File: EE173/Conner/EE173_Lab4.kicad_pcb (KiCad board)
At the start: 2 copper layers, 81.3 x 57.1 mm, 24 parts, among them J1 Conn_01x02_Male, J2 Conn_01x02_Male, J3 Test Line, J4 OSC, U1 74HC00, U2 L7806

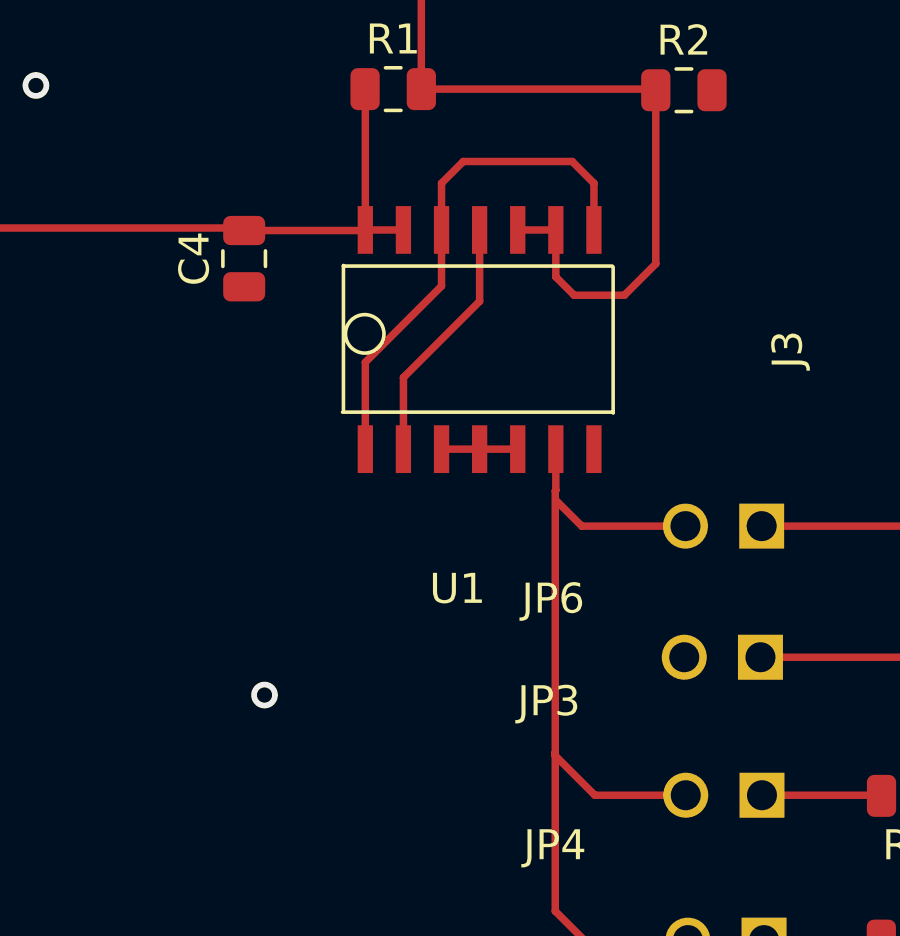
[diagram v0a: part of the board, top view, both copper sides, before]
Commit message: Nothing New
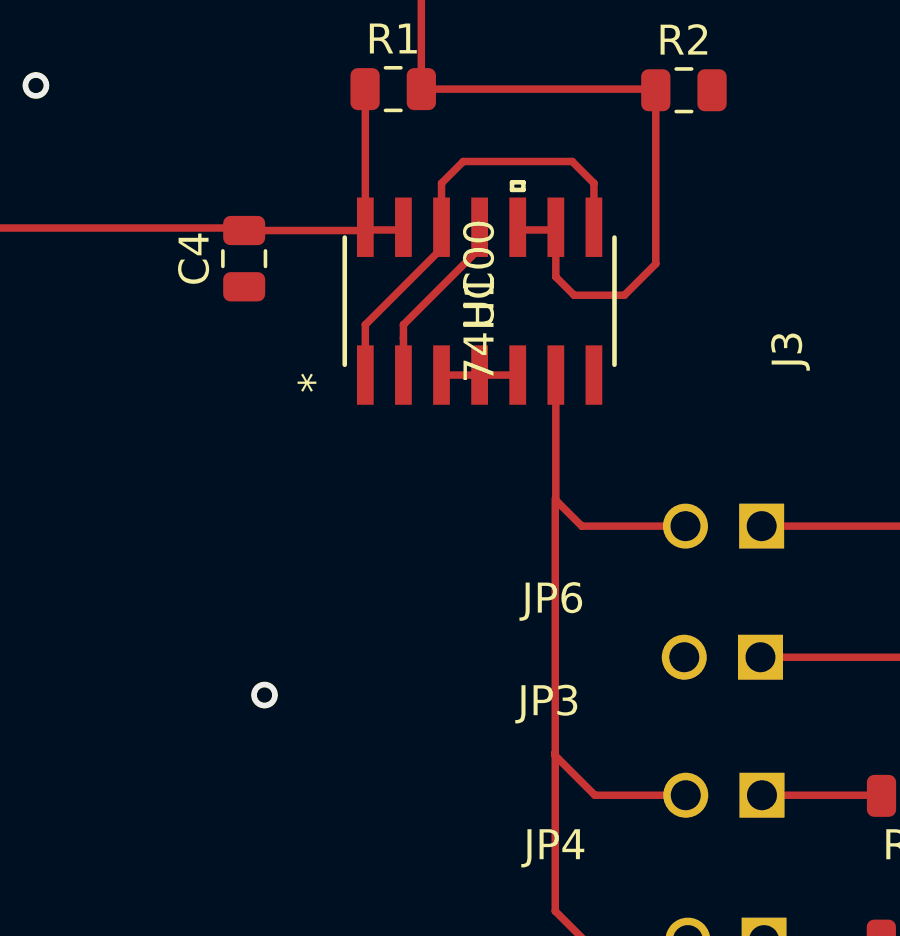
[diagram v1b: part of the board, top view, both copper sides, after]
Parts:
- U1: footprint My_Footprints:HC00 -> digikey:SN74HC00DR
- moved U1 5.37 mm to (241.5, 61.4), turned to 90 degrees
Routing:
- net Net-(JP4-Pad1): track 29.9 -> 32.4 mm
- net Net-(U1-Pad11): track 8.36 -> 5.98 mm
- net Net-(U1-Pad1): track 17.2 -> 14.8 mm
